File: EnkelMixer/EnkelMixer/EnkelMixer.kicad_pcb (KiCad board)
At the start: 2 copper layers, 62.9 x 115.6 mm, 73 parts, among them J1 PJ301M-12, J10 PJ301M-12, J2 PJ301M-12, J3 PJ301M-12, J4 PJ301M-12, J5 PJ301M-12, J6 PJ301M-12, J7 PJ301M-12, J8 PJ301M-12, J9 PJ301M-12, U1 TL074

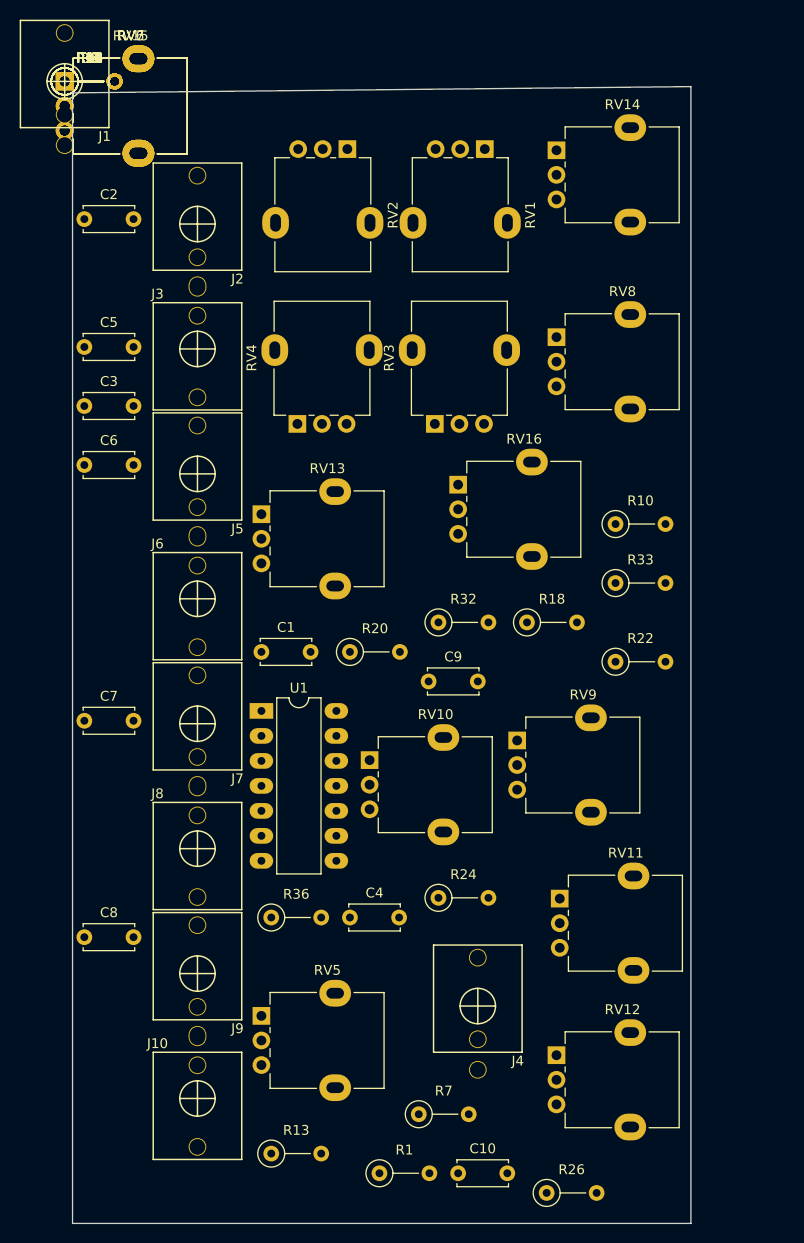
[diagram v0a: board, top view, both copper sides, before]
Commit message: hmm
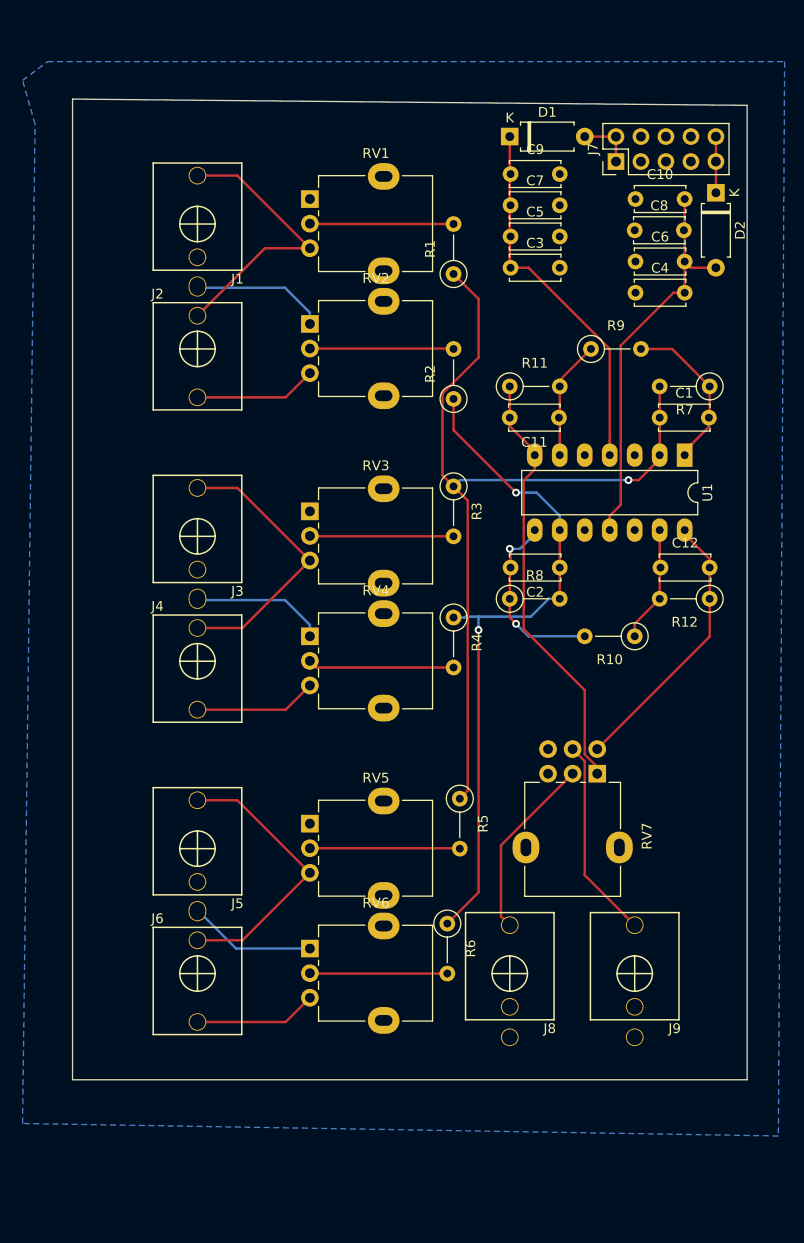
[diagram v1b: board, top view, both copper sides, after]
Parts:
- removed J10: PJ301M-12, eurorack:PJ301M-12
- removed R13, R14, R15, R16, R17, R18, R19, R20, R21, R22, R23, R24, R25, R26, R27, R28, R29, R30, R31, R32, R33, R34, R35, R36: 1K, Resistor_THT:R_Axial_DIN0207_L6.3mm_D2.5mm_P5.08mm_Vertical
- removed RV10, RV11, RV12, RV13, RV14, RV15, RV16, RV8, RV9: 10K, Potentiometer_THT:Potentiometer_Alpha_RD901F-40-00D_Single_Vertical
- added C11: 10pF, Capacitor_THT:C_Disc_D5.0mm_W2.5mm_P5.00mm, F.Cu at (227.2, 83.2)
- added C12: 10pF, Capacitor_THT:C_Disc_D5.0mm_W2.5mm_P5.00mm, F.Cu at (237.6, 98.4)
- added D1: D, Diode_THT:D_A-405_P7.62mm_Horizontal, F.Cu at (222.2, 54.6)
- added D2: D, Diode_THT:D_A-405_P7.62mm_Horizontal, F.Cu at (243.2, 60.3)
- C1: value 22pF -> 10pF
- C10, C9: value 0.1uF -> 10uF
- C2: value 0.1uF -> 10pF
- C3, C5, C6, C7, C8: value 0.1uF -> 100nF
- C4: value 22pF -> 100nF
- J1: value PJ301M-12 -> IN1L
- J2: value PJ301M-12 -> IN1R
- J3: value PJ301M-12 -> IN2L
- J4: value PJ301M-12 -> IN2R
- J5: value PJ301M-12 -> IN3L
- J6: value PJ301M-12 -> IN3R
- J7: value PJ301M-12 -> EURO_PWR_2x5; footprint eurorack:PJ301M-12 -> Connector_PinHeader_2.54mm:PinHeader_2x05_P2.54mm_Vertical
- J8: value PJ301M-12 -> OUT-L
- J9: value PJ301M-12 -> OUT-R
- R1, R10, R11, R2, R3, R4, R5, R7, R8, R9: value 1K -> 10K
- R12, R6: value 39K -> 10K
- RV1, RV2, RV3, RV4, RV5, RV6: value 10K -> 100K
- RV7: value 10K -> R_POT_Dual_Separate; footprint Potentiometer_THT:Potentiometer_Alpha_RD901F-40-00D_Single_Vertical -> Potentiometer_THT:Potentiometer_Alpha_RD902F-40-00D_Dual_Vertical
- moved C10 100.7 mm to (235.0, 61.0)
- moved R6 94.0 mm to (215.9, 134.6), turned to 270 degrees
- moved R1 91.7 mm to (216.5, 68.6), turned to 90 degrees
- moved RV6 91.6 mm to (201.9, 137.2)
- moved C8 91.1 mm to (234.9, 64.1)
- moved RV7 88.8 mm to (231.1, 119.4), turned to 270 degrees
- moved R12 84.1 mm to (242.6, 101.6), turned to 180 degrees
- moved R5 83.3 mm to (217.2, 121.9), turned to 270 degrees
- moved R7 79.7 mm to (242.6, 80.0), turned to 180 degrees
- moved J7 71.2 mm to (233.0, 57.1), turned to 90 degrees
- moved C4 69.8 mm to (235.0, 70.5)
- moved R8 69.4 mm to (222.2, 101.6)
- moved C7 68.0 mm to (222.3, 61.6)
- moved R4 67.3 mm to (216.5, 103.5), turned to 270 degrees
- moved R9 60.0 mm to (230.5, 76.2)
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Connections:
- C10 pad 1: Net-(C10-Pad1) -> Earth
- C10 pad 2: Net-(C10-Pad2) -> -12V
- C2 pad 1: Net-(C2-Pad1) -> Right
- C3 pad 1: Net-(C3-Pad1) -> +12V
- C3 pad 2: Net-(C3-Pad2) -> Earth
- C4 pad 1: Right -> Earth
- C4 pad 2: Net-(C4-Pad2) -> -12V
- C5 pad 1: Net-(C5-Pad1) -> +12V
- C5 pad 2: Net-(C5-Pad2) -> Earth
- C6 pad 1: Net-(C6-Pad1) -> Earth
- C6 pad 2: Net-(C6-Pad2) -> -12V
- C7 pad 1: Net-(C7-Pad1) -> +12V
- C7 pad 2: Net-(C7-Pad2) -> Earth
- C8 pad 1: Net-(C8-Pad1) -> Earth
- C8 pad 2: Net-(C8-Pad2) -> -12V
- C9 pad 1: Net-(C9-Pad1) -> +12V
- C9 pad 2: Net-(C9-Pad2) -> Earth
- J1 pad 2: Earth -> Net-(J1-Pad2)
- J1 pad 3: Net-(J1-Pad3) -> Mono1
- J2 pad 2: Earth -> Mono1
- J2 pad 3: Net-(C2-Pad1) -> Net-(J2-Pad3)
- J3 pad 2: Earth -> Net-(J3-Pad2)
- J3 pad 3: Net-(C3-Pad1) -> Mono2
- J4 pad 2: Earth -> Mono2
- J5 pad 2: Earth -> Net-(J5-Pad2)
- J5 pad 3: Net-(C5-Pad1) -> Mono3
- J6 pad 2: Earth -> Mono3
- J6 pad 3: Net-(C6-Pad1) -> Net-(J6-Pad3)
- J7 pad 1: Earth -> Net-(D1-Pad2)
- J7 pad 2: Earth -> Net-(D1-Pad2)
- J7 pad 3: Net-(C7-Pad1) -> Earth
- J8 pad 2: Earth -> Net-(J8-Pad2)
- J8 pad 3: Net-(C8-Pad1) -> Net-(J8-Pad3)
- J9 pad 2: Earth -> Net-(J9-Pad2)
- J9 pad 3: Net-(C9-Pad1) -> Net-(J9-Pad3)
- R1 pad 1: Net-(R1-Pad1) -> Left
- R10 pad 1: Right -> Net-(C12-Pad1)
- R10 pad 2: Net-(R10-Pad2) -> Net-(C2-Pad2)
- R11 pad 1: Net-(J4-Pad3) -> Net-(C11-Pad2)
- R11 pad 2: Net-(C4-Pad2) -> Net-(C11-Pad1)
- R12 pad 1: Net-(C4-Pad2) -> Net-(C12-Pad2)
- R12 pad 2: Right -> Net-(C12-Pad1)
- R2 pad 1: Left -> Right
- R2 pad 2: Net-(R1-Pad1) -> Net-(R2-Pad2)
- R3 pad 1: Net-(J1-Pad3) -> Left
- R3 pad 2: Net-(C1-Pad2) -> Net-(R3-Pad2)
- R4 pad 1: Net-(R4-Pad1) -> Right
- R4 pad 2: Net-(R1-Pad2) -> Net-(R4-Pad2)
- R5 pad 1: Right -> Left
- R5 pad 2: Net-(R4-Pad1) -> Net-(R5-Pad2)
- R6 pad 1: Net-(C1-Pad2) -> Right
- R6 pad 2: Left -> Net-(R6-Pad2)
- R7 pad 1: Net-(R7-Pad1) -> Net-(C1-Pad2)
- R7 pad 2: Net-(R7-Pad2) -> Left
- R8 pad 1: Left -> Net-(C2-Pad2)
- R8 pad 2: Net-(R7-Pad1) -> Right
- R9 pad 1: Net-(R10-Pad2) -> Net-(C11-Pad1)
- R9 pad 2: Net-(R7-Pad2) -> Net-(C1-Pad2)
- RV1 pad 1: Net-(R1-Pad1) -> Earth
- RV1 pad 2: Earth -> Net-(R1-Pad2)
- RV1 pad 3: Net-(R4-Pad1) -> Mono1
- RV2 pad 2: Net-(R1-Pad2) -> Net-(R2-Pad2)
- RV2 pad 3: Net-(C2-Pad2) -> Net-(J2-Pad3)
- RV3 pad 1: Net-(R7-Pad1) -> Earth
- RV3 pad 2: Earth -> Net-(R3-Pad2)
- RV3 pad 3: Net-(R10-Pad2) -> Mono2
- RV4 pad 2: Net-(R7-Pad2) -> Net-(R4-Pad2)
- RV4 pad 3: Net-(C3-Pad2) -> Net-(J4-Pad3)
- RV5 pad 1: Net-(R13-Pad1) -> Earth
- RV5 pad 2: Earth -> Net-(R5-Pad2)
- RV5 pad 3: Net-(R15-Pad1) -> Mono3
- RV6 pad 2: Net-(R13-Pad2) -> Net-(R6-Pad2)
- RV6 pad 3: Net-(C5-Pad2) -> Net-(J6-Pad3)
- RV7 pad 1: Net-(R17-Pad1) -> Net-(C11-Pad2)
- RV7 pad 2: Earth -> Net-(J8-Pad3)
- RV7 pad 3: Net-(R19-Pad1) -> Earth
- U1 pad 10: Net-(U1-Pad10) -> Earth
- U1 pad 11: Net-(U1-Pad11) -> -12V
- U1 pad 12: Net-(U1-Pad12) -> Earth
- U1 pad 13: Net-(U1-Pad13) -> Net-(C12-Pad1)
- U1 pad 14: Net-(U1-Pad14) -> Net-(C12-Pad2)
- U1 pad 4: Net-(U1-Pad4) -> +12V
- U1 pad 6: Right -> Net-(C11-Pad1)
- U1 pad 7: Net-(C4-Pad2) -> Net-(C11-Pad2)
- U1 pad 8: Net-(U1-Pad8) -> Net-(C2-Pad2)
- U1 pad 9: Net-(U1-Pad9) -> Right
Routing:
- net Left: track 0.00 -> 86.8 mm, vias 0 -> 1
- net Right: track 0.00 -> 70.2 mm, vias 0 -> 2
- net Net-(C11-Pad2): track 0.00 -> 44.0 mm
- net -12V: track 0.00 -> 41.0 mm
- net Earth: track 0.00 -> 40.3 mm
- net +12V: track 0.00 -> 37.7 mm
- net Mono3: track 0.00 -> 28.8 mm
- net Mono2: track 0.00 -> 28.8 mm
- net Mono1: track 0.00 -> 28.8 mm
- net Net-(C12-Pad2): track 0.00 -> 28.1 mm
- net Net-(J9-Pad3): track 0.00 -> 20.5 mm
- net Net-(C2-Pad2): track 0.00 -> 19.0 mm, vias 0 -> 2
- net Net-(J8-Pad3): track 0.00 -> 18.8 mm
- net Net-(C1-Pad2): track 0.00 -> 16.6 mm
- net Net-(R5-Pad2): track 0.00 -> 15.3 mm
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- added copper zone on B.Cu, net Earth
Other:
- board size 62.9 x 115.6 mm -> 68.6 x 99.7 mm
